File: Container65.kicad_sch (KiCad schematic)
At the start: 88 parts, among them J1 Conn_01x03, J2 Conn_01x06, U1 RP2040, U2 TYPE-C-31-M-12, U3 XC6206PxxxMR, U4 W25Q128JVS, U5 USB Boot, U6 Reset, Y1 12MHz - 20pF

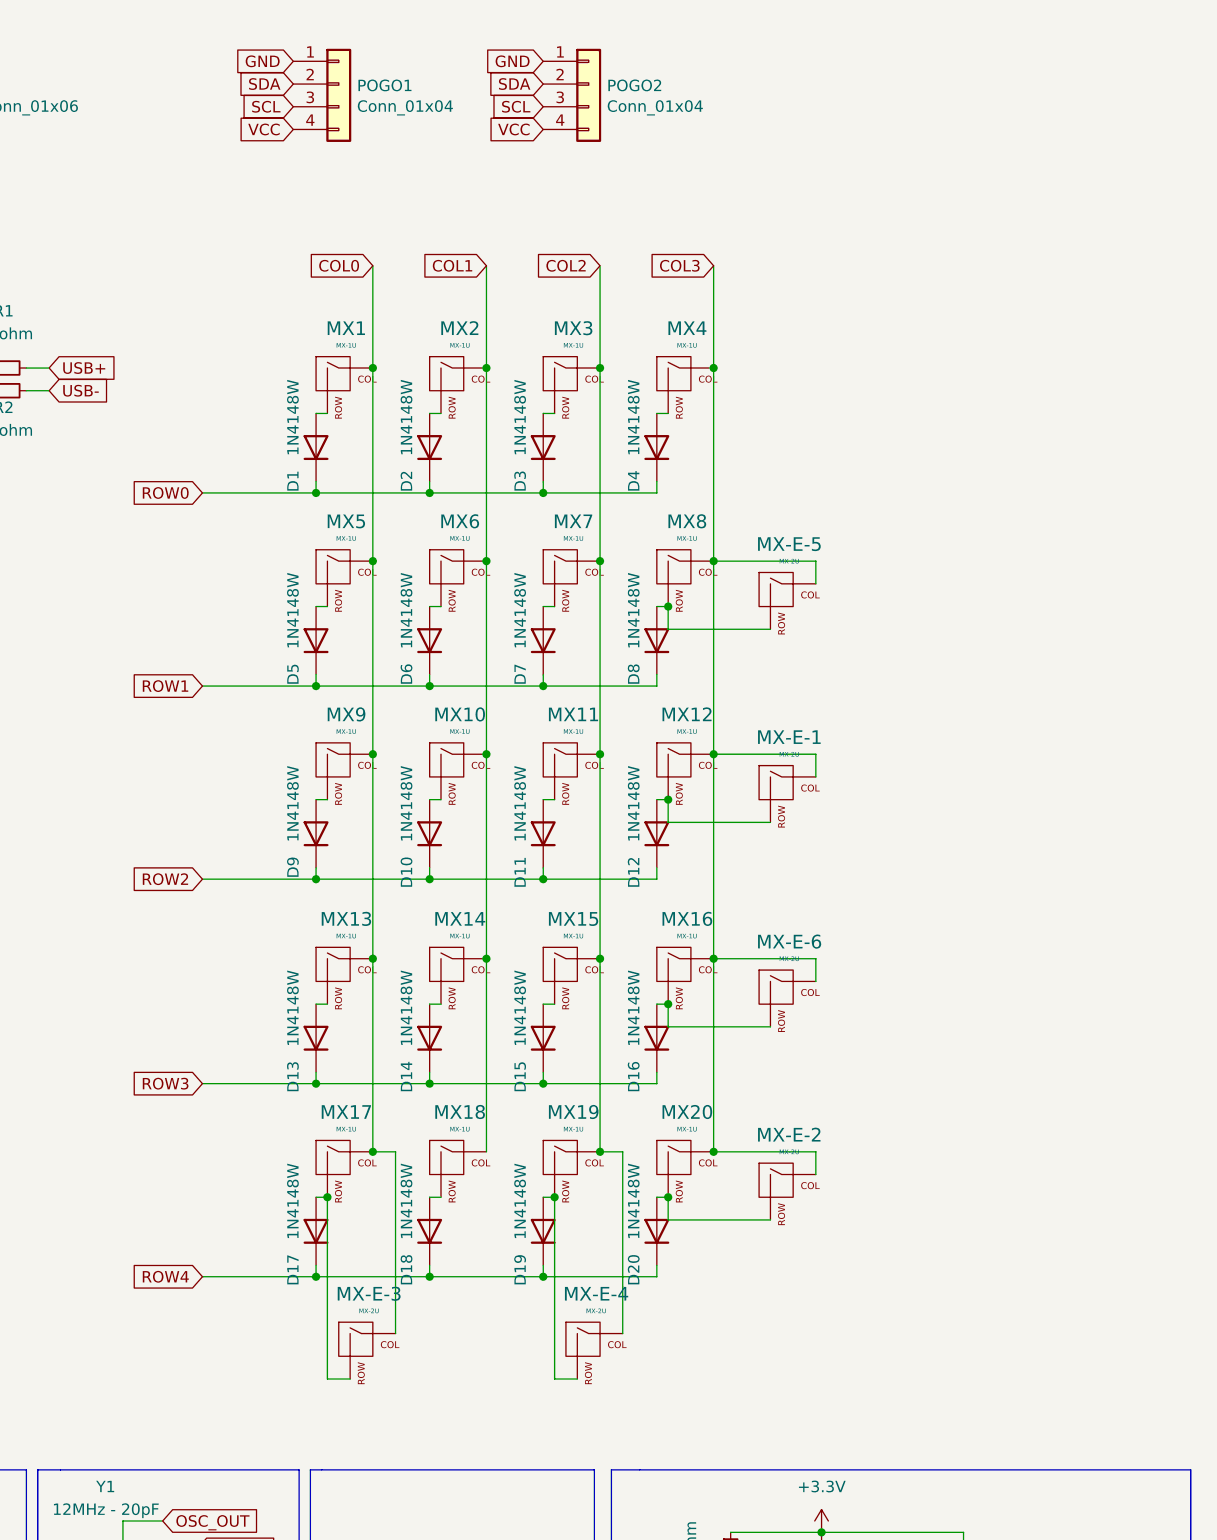
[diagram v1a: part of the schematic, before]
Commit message: Design
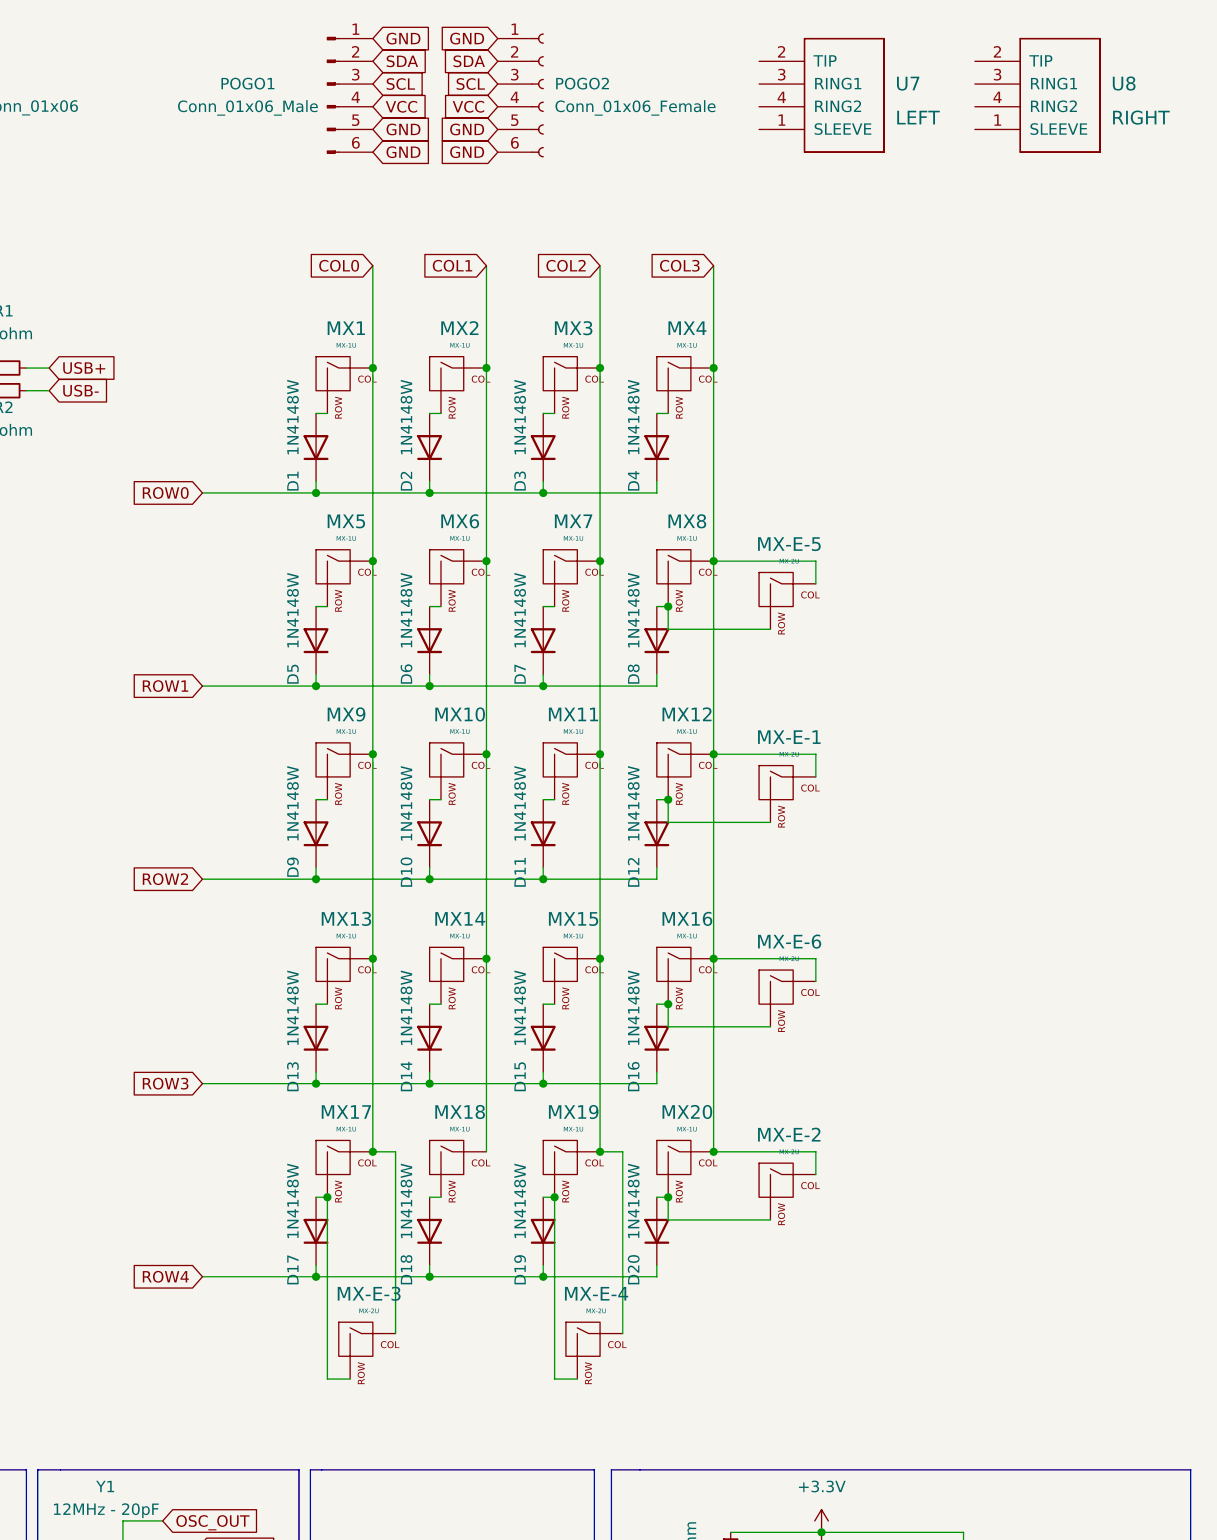
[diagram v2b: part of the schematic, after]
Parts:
- removed POGO1: Conn_01x04, 65Numpad:PogoConnector, symbol Connector_Generic:Conn_01x04
- removed POGO2: Conn_01x04, 65Numpad:PogoConnectorMirrored, symbol Connector_Generic:Conn_01x04
- added POGO1: Conn_01x06_Male, extras:1x04_3.00mm_Magnetic Pogo_Male, symbol Connector:Conn_01x06_Male
- added POGO2: Conn_01x06_Female, extras:1x04_3.00mm_Magnetic Pogo_Female_2, symbol Connector:Conn_01x06_Female
- added U7: LEFT, Keebio-Parts:TRRS-PJ-320A, symbol keebio:TRRS
- added U8: RIGHT, Keebio-Parts:TRRS-PJ-320A, symbol keebio:TRRS
- C1, C10, C11, C12, C13, C14, C15, C16, C17, C18, C2, C3, C4, C5, C6, C7, C8, C9: footprint Capacitor_SMD:C_0402_1005Metric -> Keebio-Parts:C_0402
- D1, D10, D11, D12, D13, D14, D15, D16, D17, D18, D19, D2, D20, D21, D3, D4, D5, D6, D7, D8, D9: footprint Diode_SMD:D_SOD-123 -> Keebio-Parts:D_SOD123
- D22: footprint LED_SMD:LED_0805_2012Metric -> Keebio-Parts:R_0805
- F1: footprint Fuse:Fuse_0805_2012Metric -> Keebio-Parts:Fuse_0805
- MX-E-1, MX-E-2, MX-E-3, MX-E-4, MX-E-5, MX-E-6: footprint MX_Only:MXOnly-1U-NoLEDHotswap -> Switch_Keyboard_Hotswap_Kailh:SW_Hotswap_Kailh_MX_1.00u_Extras
- MX1, MX10, MX11, MX12, MX13, MX14, MX15, MX16, MX17, MX18, MX19, MX2, MX20, MX3, MX4, MX5, MX6, MX7, MX8, MX9: footprint MX_Only:MXOnly-1U-NoLEDHotswap -> Switch_Keyboard_Hotswap_Kailh:SW_Hotswap_Kailh_MX_1.00u_Modified
- R1, R2: footprint Resistor_SMD:R_0603_1608Metric -> Keebio-Parts:R_0402
- R3, R4, R5, R6, R7, R8, R9: footprint Resistor_SMD:R_0402_1005Metric -> Keebio-Parts:R_0402
- U1: footprint footprints:rp2040 -> extras:rp2040
- U2: footprint footprints:simple-usb-c -> extras:simple-usb-c
- U5, U6: footprint footprints:tactile-switch -> extras:tactile-switch
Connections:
- net GND: now also POGO1.1 (Pin_1), POGO1.5 (Pin_5), POGO1.6 (Pin_6), POGO2.1 (Pin_1), POGO2.5 (Pin_5), POGO2.6 (Pin_6)
- net SCL: now also POGO1.3 (Pin_3), POGO2.3 (Pin_3)
- net SDA: now also POGO1.2 (Pin_2), POGO2.2 (Pin_2)
- net VCC: now also POGO1.4 (Pin_4), POGO2.4 (Pin_4)

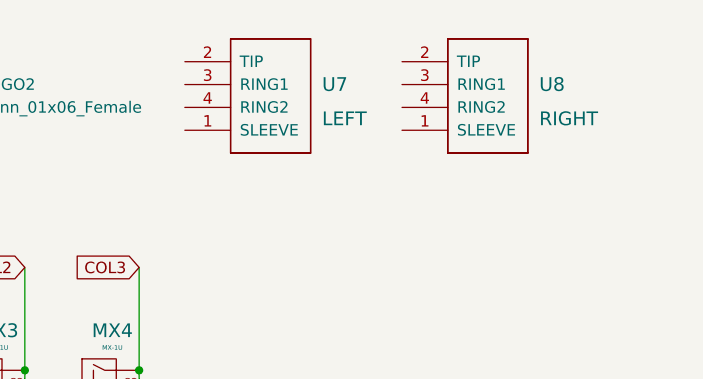
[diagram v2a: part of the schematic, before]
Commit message: Copy from backup
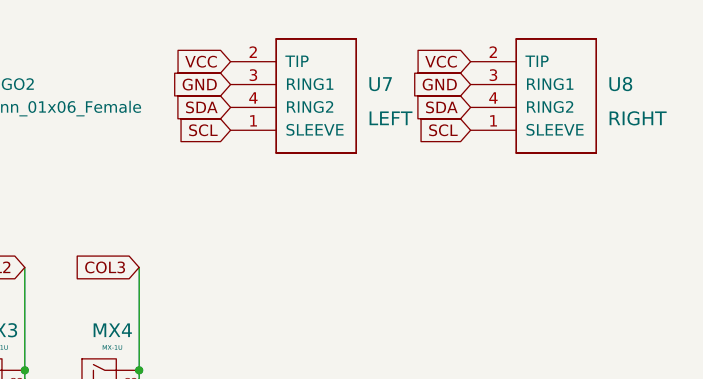
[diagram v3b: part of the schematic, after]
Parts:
- U7, U8: footprint Keebio-Parts:TRRS-PJ-320A -> Keebio-Parts:TRRS-PJ-320D
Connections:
- net GND: now also U7.3 (RING1), U8.3 (RING1)
- net SCL: now also U7.1 (SLEEVE), U8.1 (SLEEVE)
- net SDA: now also U7.4 (RING2), U8.4 (RING2)
- net VCC: now also U7.2 (TIP), U8.2 (TIP)
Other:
- moved on the sheet: U7, U8
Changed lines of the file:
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@@
+    )
+  )
+  (global_label "VCC" (shape input) (at 248.92 20.32 180)
+    (effects (font (size 1.27 1.27)) (justify right))
+    (property "Intersheet References" "${INTERSHEET_REFS}" (id 0) (at -158.75 -7.62 0)
+      (effects (font (size 1.27 1.27)) hide)
     )
   )
@@
     )
   )
+  (global_label "GND" (shape input) (at 222.25 22.86 180)
+    (effects (font (size 1.27 1.27)) (justify right))
+    (property "Intersheet References" "${INTERSHEET_REFS}" (id 0) (at -185.42 -2.54 0)
+      (effects (font (size 1.27 1.27)) hide)
+    )
+  )
   (global_label "XOUT_MCU" (shape input) (at 42.545 105.41 270) (fields_autoplaced)
     (effects (font (size 1.27 1.27)) (justify right))
@@
     )
   )
+  (global_label "SCL" (shape input) (at 222.25 27.94 180) (fields_autoplaced)
+    (effects (font (size 1.27 1.27)) (justify right))
+    (property "Intersheet References" "${INTERSHEET_REFS}" (id 0) (at 377.19 187.96 0)
+      (effects (font (size 1.27 1.27)) hide)
+    )
+  )
   (global_label "QSPI_SD3" (shape input) (at 50.8 77.47 180) (fields_autoplaced)
     (effects (font (size 1.27 1.27)) (justify right))
@@
     )
   )
+  (global_label "VCC" (shape input) (at 222.25 20.32 180)
+    (effects (font (size 1.27 1.27)) (justify right))
+    (property "Intersheet References" "${INTERSHEET_REFS}" (id 0) (at -185.42 -7.62 0)
+      (effects (font (size 1.27 1.27)) hide)
+    )
+  )
   (global_label "QSPI_SCLK" (shape input) (at 50.8 81.28 180) (fields_autoplaced)
     (effects (font (size 1.27 1.27)) (justify right))
@@
     )
   )
+  (global_label "SCL" (shape input) (at 248.92 27.94 180) (fields_autoplaced)
+    (effects (font (size 1.27 1.27)) (justify right))
+    (property "Intersheet References" "${INTERSHEET_REFS}" (id 0) (at 403.86 187.96 0)
+      (effects (font (size 1.27 1.27)) hide)
+    )
+  )
   (global_label "CLM1" (shape input) (at 114.3 105.41 0) (fields_autoplaced)
     (effects (font (size 1.27 1.27)) (justify left))
@@
     )
   )
+  (global_label "SDA" (shape input) (at 222.25 25.4 180) (fields_autoplaced)
+    (effects (font (size 1.27 1.27)) (justify right))
+    (property "Intersheet References" "${INTERSHEET_REFS}" (id 0) (at 377.19 182.88 0)
+      (effects (font (size 1.27 1.27)) hide)
+    )
+  )
   (global_label "QSPI_SS" (shape input) (at 178.435 217.17 180) (fields_autoplaced)
     (effects (font (size 1.27 1.27)) (justify right))
@@
     )
   )
+  (global_label "GND" (shape input) (at 248.92 22.86 180)
+    (effects (font (size 1.27 1.27)) (justify right))
+    (property "Intersheet References" "${INTERSHEET_REFS}" (id 0) (at -158.75 -2.54 0)
+      (effects (font (size 1.27 1.27)) hide)
+    )
+  )
   (global_label "CC1" (shape input) (at 52.705 207.01 0) (fields_autoplaced)
     (effects (font (size 1.27 1.27)) (justify left))
@@
     (property "Intersheet References" "${INTERSHEET_REFS}" (id 0) (at 121.6721 95.3294 0)
       (effects (font (size 1.27 1.27)) (justify left) hide)
+    )
+  )
+  (global_label "SDA" (shape input) (at 248.92 25.4 180) (fields_autoplaced)
+    (effects (font (size 1.27 1.27)) (justify right))
+    (property "Intersheet References" "${INTERSHEET_REFS}" (id 0) (at 403.86 182.88 0)
+      (effects (font (size 1.27 1.27)) hide)
     )
   )
@@
     (pin "2")
   )
-  (symbol (lib_id "keebio:TRRS") (at 226.06 30.48 0) (unit 1)
-    (in_bom yes) (on_board yes) (fields_autoplaced)
-    (property "Reference" "U7" (id 0) (at 232.41 22.86 0)
+  (symbol (lib_id "keebio:TRRS") (at 231.14 30.48 0) (unit 1)
+    (in_bom yes) (on_board yes) (fields_autoplaced)
+    (property "Reference" "U7" (id 0) (at 237.49 22.86 0)
       (effects (font (size 1.524 1.524)) (justify left))
     )
-    (property "Value" "LEFT" (id 1) (at 232.41 26.67 0)
+    (property "Value" "LEFT" (id 1) (at 237.49 26.67 0)
       (effects (font (size 1.524 1.524)) (justify left))
     )
-    (property "Footprint" "Keebio-Parts:TRRS-PJ-320A" (id 2) (at 229.87 30.48 0)
-      (effects (font (size 1.524 1.524)) hide)
-    )
-    (property "Datasheet" "" (id 3) (at 229.87 30.48 0)
+    (property "Footprint" "Keebio-Parts:TRRS-PJ-320D" (id 2) (at 234.95 30.48 0)
+      (effects (font (size 1.524 1.524)) hide)
+    )
+    (property "Datasheet" "" (id 3) (at 234.95 30.48 0)
       (effects (font (size 1.524 1.524)) hide)
     )
@@
     (pin "2")
   )
-  (symbol (lib_id "keebio:TRRS") (at 250.19 30.48 0) (unit 1)
-    (in_bom yes) (on_board yes) (fields_autoplaced)
-    (property "Reference" "U8" (id 0) (at 256.54 22.86 0)
+  (symbol (lib_id "keebio:TRRS") (at 257.81 30.48 0) (unit 1)
+    (in_bom yes) (on_board yes) (fields_autoplaced)
+    (property "Reference" "U8" (id 0) (at 264.16 22.86 0)
       (effects (font (size 1.524 1.524)) (justify left))
     )
-    (property "Value" "RIGHT" (id 1) (at 256.54 26.67 0)
+    (property "Value" "RIGHT" (id 1) (at 264.16 26.67 0)
       (effects (font (size 1.524 1.524)) (justify left))
     )
-    (property "Footprint" "Keebio-Parts:TRRS-PJ-320A" (id 2) (at 254 30.48 0)
-      (effects (font (size 1.524 1.524)) hide)
-    )
-    (property "Datasheet" "" (id 3) (at 254 30.48 0)
+    (property "Footprint" "Keebio-Parts:TRRS-PJ-320D" (id 2) (at 261.62 30.48 0)
+      (effects (font (size 1.524 1.524)) hide)
+    )
+    (property "Datasheet" "" (id 3) (at 261.62 30.48 0)
       (effects (font (size 1.524 1.524)) hide)
     )
@@
     )
     (path "/98c150b7-049e-4fac-8f45-60f2576a64f5"
-      (reference "U7") (unit 1) (value "LEFT") (footprint "Keebio-Parts:TRRS-PJ-320A")
+      (reference "U7") (unit 1) (value "LEFT") (footprint "Keebio-Parts:TRRS-PJ-320D")
     )
     (path "/bc53684d-e6be-49c8-ab37-fbed73b271a0"
-      (reference "U8") (unit 1) (value "RIGHT") (footprint "Keebio-Parts:TRRS-PJ-320A")
+      (reference "U8") (unit 1) (value "RIGHT") (footprint "Keebio-Parts:TRRS-PJ-320D")
     )
     (path "/3d1b2c07-f701-4a6d-98db-4deeb93d797f"
